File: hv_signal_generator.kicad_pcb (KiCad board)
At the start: 2 copper layers, 83.8 x 121.9 mm, 210 parts, among them IC1 ATMEG328PU, J1 CONN_4, J2 CONN_10, J3 CONN_2, J4 CONN_2, J5 CONN_40, P1 CONN_6, P2 CONN_6, SW1 DPST, U1 74HC595A, U2 74HC595A, U3 74HC595A, U4 74HC595A, U5 74HC595A, U6 7400, X1 16MHz

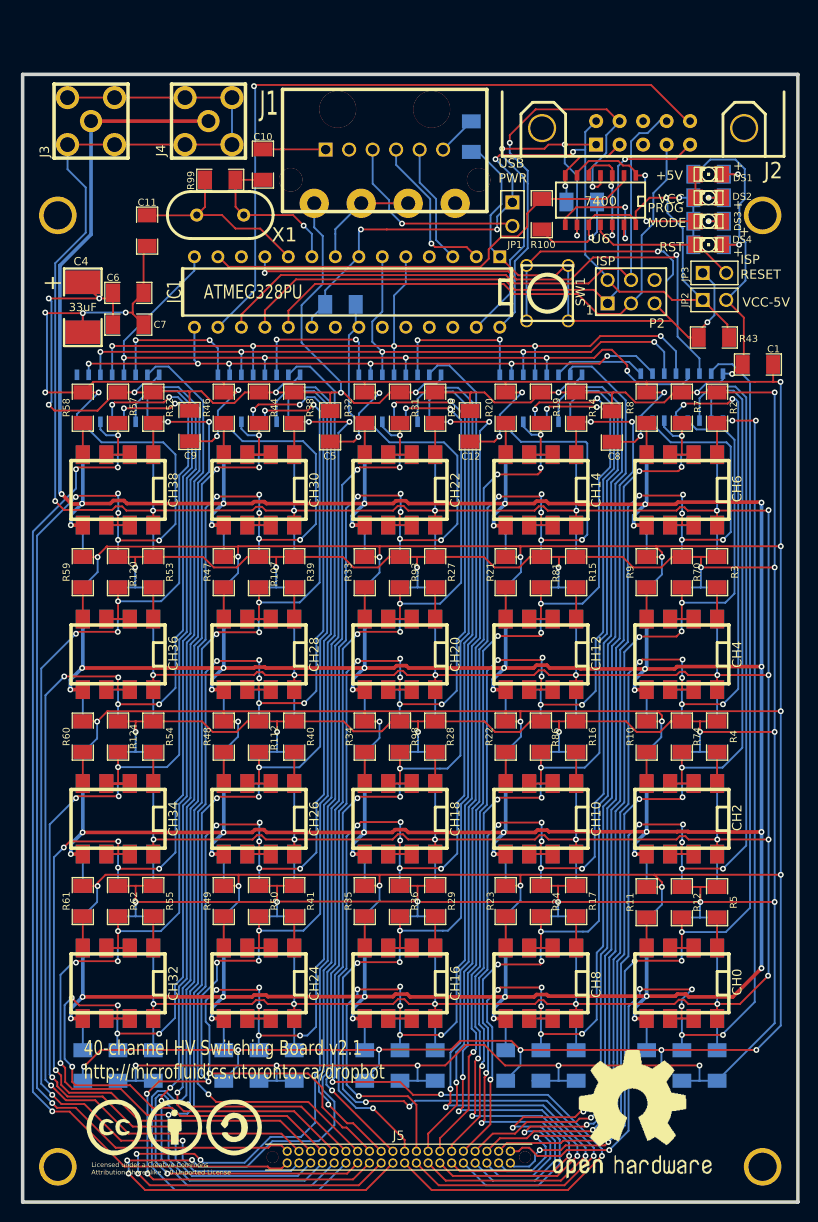
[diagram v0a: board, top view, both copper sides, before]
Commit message: Complete layout
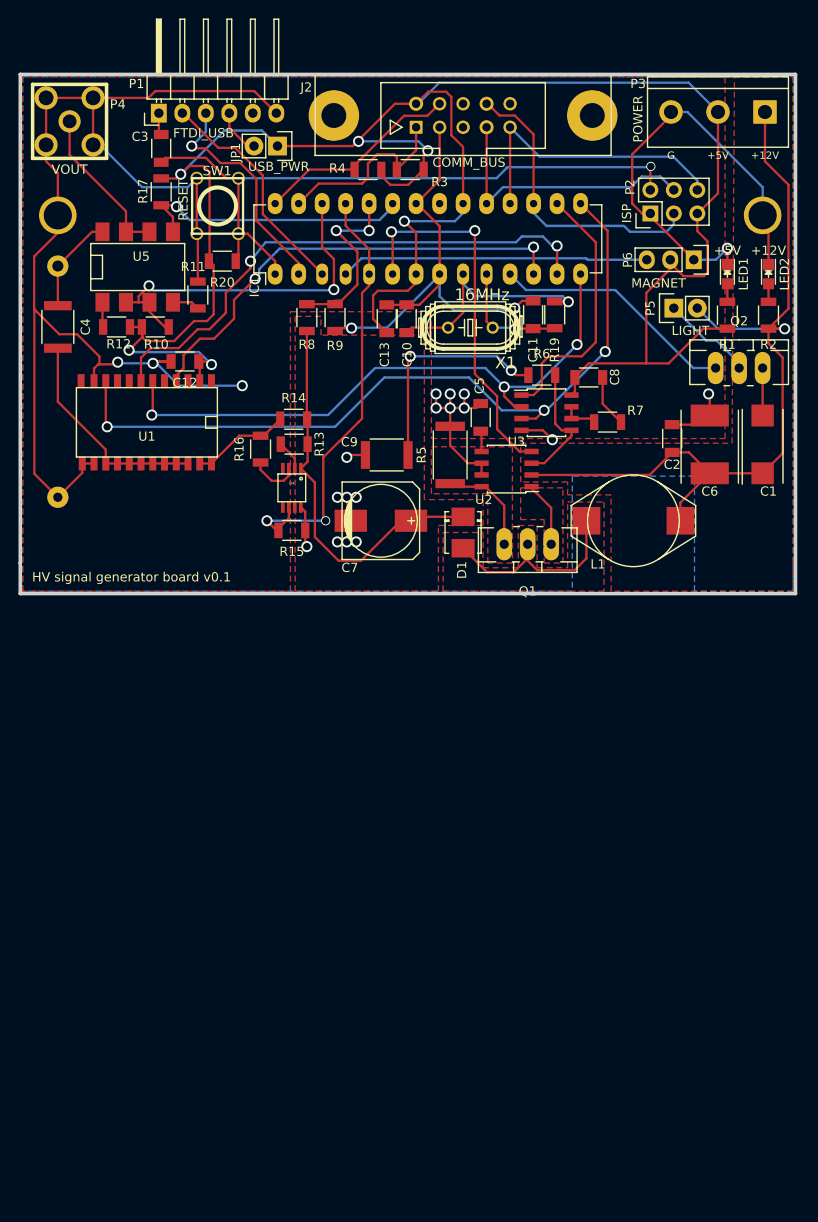
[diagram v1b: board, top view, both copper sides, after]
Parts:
- removed the 1PIN at (20.3, 133.3)
- removed the 1PIN at (96.5, 133.3)
- removed C14: 0.1uF, SM1206
- removed CH0, CH1, CH10, CH11, CH12, CH13, CH14, CH15, CH16, CH17, CH18, CH19, CH2, CH20, CH21, CH22, CH23, CH24, CH25, CH26, CH27, CH28, CH29, CH3, CH30, CH31, CH32, CH33, CH34, CH35, CH36, CH37, CH38, CH39, CH4, CH5, CH6, CH7, CH8, CH9: AQW216, 8DIPCMS
- removed DS1: +5V, LED-1206
- removed DS2: VCC, LED-1206
- removed DS3: PROG_MODE, LED-1206
- removed DS4: RST, LED-1206
- removed G***: LOGO, CC_A_SA_LOGO
- removed G***: LOGO, OSHWLOGO0.75IN
- removed J1: CONN_4, Molex_15-24-4441
- removed J3, J4: CONN_2, JACK_SMA
- removed J5: CONN_40, TFML-120-01-XXX-D-RA
- removed JP2: JUMPER, PIN_ARRAY_2X1
- removed JP3: ISP RESET, PIN_ARRAY_2X1
- removed R100, R125, R126, R127, R45: 1k, SM1206
- removed R101, R106, R107, R112, R114, R118, R120, R124, R24, R25, R30, R31, R36, R37, R42, R44, R50, R51, R56, R57, R62, R64, R68, R70, R74, R75, R80, R81, R86, R87, R92, R93, R98: 4.75k, SM1206
- removed R102, R103, R104, R105, R108, R109, R110, R111, R113, R115, R116, R117, R119, R121, R122, R123, R21, R22, R23, R26, R27, R28, R29, R32, R33, R34, R35, R38, R39, R40, R41, R46, R47, R48, R49, R52, R53, R54, R55, R58, R59, R60, R61, R63, R65, R66, R67, R69, R71, R72, R73, R76, R77, R78, R79, R82, R83, R84, R85, R88, R89, R90, R91, R94, R95, R96, R97: 375, SM1206
- removed R43: 10k, SM1206
- removed R99: 1Meg, SM1206
- removed U6: 7400, SO14E
- added D1: ES2F, Diodes_SMD:DO-214BA, F.Cu at (64.1, 64.8)
- added L1: 100uH, Inductors:self_cms_we-pd3, F.Cu at (82.5, 63.5)
- added LED1: +5V, LEDs:LED_0805, F.Cu at (92.7, 36.8)
- added LED2: +12V, LEDs:LED_0805, F.Cu at (97.2, 36.8)
- added P3: POWER, Connect:bornier3, F.Cu at (91.7, 19.3)
- added P4: VOUT, footprints:JACK_SMA, F.Cu at (21.6, 20.3)
- added P5: LIGHT, Pin_Headers:Pin_Header_Straight_1x02, F.Cu at (86.9, 40.5)
- added P6: MAGNET, Pin_Headers:Pin_Header_Straight_1x03, F.Cu at (89.1, 35.3)
- added Q1: IRF644PBF, TO_SOT_Packages_THT:TO-220_Neutral123_Vertical_LargePads, F.Cu at (71.1, 66.0)
- added Q2: P16NF06, TO_SOT_Packages_THT:TO-220_Neutral123_Vertical_LargePads, F.Cu at (94.0, 47.0)
- C1: value 0.1uF -> 10uF; footprint SM1206 -> Capacitors_Tantalum_SMD:TantalC_SizeD_EIA-7343_Reflow
- C10, C11, C12, C5, C8: footprint SM1206 -> Capacitors_SMD:C_1206
- C13, C3: footprint SM1206 -> Capacitors_SMD:C_1206; moved to F.Cu
- C2: value 33uF -> 0.1uF; footprint SM2917 -> Capacitors_SMD:C_1206; moved to F.Cu
- C4: value 33uF -> 0.1uF; footprint SM2917 -> Capacitors_SMD:C_1812
- C6: value 0.1uF -> 100uF,35V; footprint SM1206 -> Capacitors_Tantalum_SMD:TantalC_SizeE_EIA-7360_Reflow
- C7: value 0.01uF -> 4u7,250V; footprint SM1206 -> Capacitors_SMD:c_elec_8x10.5
- C9: value 0.1uF -> 100nF,250V; footprint SM1206 -> Capacitors_SMD:C_1812
- IC1: footprint DIP-28 -> Housings_DIP:DIP-28_W7.62mm_LongPads
- J2: value CONN_10 -> COMM_BUS; footprint HE10-10C -> Connect:he10-10d
- JP1: value JUMPER -> USB_PWR; footprint PIN_ARRAY_2X1 -> Pin_Headers:Pin_Header_Straight_1x02
- P1: value CONN_6 -> FTDI_USB; footprint PIN_ARRAY-6X1 -> Pin_Headers:Pin_Header_Angled_1x06; moved to F.Cu
- P2: value CONN_6 -> ISP; footprint pin_array_3x2 -> Pin_Headers:Pin_Header_Straight_2x03
- R1: value 4.75k -> 1k; footprint SM1206 -> Resistors_SMD:R_1206; moved to F.Cu
- R10: value 375 -> 4.75k; footprint SM1206 -> Resistors_SMD:R_1206
- R11: footprint SM1206 -> Resistors_SMD:R_1206
- R12: value 4.75k -> 375; footprint SM1206 -> Resistors_SMD:R_1206
- R13: value 4.75k -> 5k; footprint SM1206 -> Resistors_SMD:R_1206; moved to F.Cu
- R14: value 375 -> 5; footprint SM1206 -> Resistors_SMD:R_1206
- R15, R17: value 375 -> 50k; footprint SM1206 -> Resistors_SMD:R_1206
- R16: value 375 -> 100k; footprint SM1206 -> Resistors_SMD:R_1206
- R18: value 4.75k -> 10k; footprint SM1206 -> Resistors_ThroughHole:Resistor_Horizontal_RM25mm
- R19: value 4.75k -> 1Meg; footprint SM1206 -> Resistors_SMD:R_1206
- R2: value 375 -> 2k; footprint SM1206 -> Resistors_SMD:R_1206
- R20: value 375 -> 10k; footprint SM1206 -> Resistors_SMD:R_1206
- R3, R4: value 375 -> 5.1k; footprint SM1206 -> Resistors_SMD:R_1206
- R5: value 375 -> 50m; footprint SM1206 -> Resistors_SMD:R_2512
- R6: value 4.75k -> 2M; footprint SM1206 -> Resistors_SMD:R_1206; moved to F.Cu
- R7: value 4.75k -> 10k; footprint SM1206 -> Resistors_SMD:R_1206
- R8: value 375 -> 2M; footprint SM1206 -> Resistors_SMD:R_1206
- R9: value 375 -> 40k; footprint SM1206 -> Resistors_SMD:R_1206
- SW1: value DPST -> RESET; footprint SW_PUSH_6mm -> footprints:SW_PUSH_6mm
- U1: value 74HC595A -> HV513; footprint SO16E -> footprints:SOW-24; moved to F.Cu
- U2: value 74HC595A -> MAX1771; footprint SO16E -> Housings_SOIC:SOIC-8_3.9x4.9mm_Pitch1.27mm; moved to F.Cu
- U3: value 74HC595A -> MCP41050; footprint SO16E -> Housings_SOIC:SOIC-8_3.9x4.9mm_Pitch1.27mm; moved to F.Cu
- U4: value 74HC595A -> HV7802; footprint SO16E -> footprints:MSOP-8; moved to F.Cu
- U5: value 74HC595A -> AQW216; footprint SO16E -> SMD_Packages:DIP-8_SMD; moved to F.Cu
- X1: footprint HC-49V -> footprints:SparkFun-HC49U-V
- moved R17 88.8 mm to (31.5, 27.9), turned to 270 degrees
- moved R12 87.2 mm to (26.7, 42.5), turned to 0 degrees
- moved R11 81.6 mm to (35.5, 39.1)
- moved R4 72.0 mm to (53.8, 25.5), turned to 180 degrees
- moved R10 69.2 mm to (30.9, 42.5), turned to 0 degrees
- moved C2 65.3 mm to (86.7, 54.6), turned to 90 degrees
- moved C6 65.0 mm to (90.8, 55.2), turned to 90 degrees
- moved R1 63.7 mm to (92.7, 41.3)
- moved R18 58.3 mm to (20.3, 61.0)
- moved U1 57.9 mm to (29.9, 52.9)
- moved R5 56.3 mm to (62.7, 56.4)
- moved R13 56.1 mm to (45.9, 55.2), turned to 180 degrees
- moved R3 54.7 mm to (58.4, 25.5), turned to 180 degrees
- moved R16 46.2 mm to (42.2, 55.8)
- moved R9 43.5 mm to (50.3, 41.5), turned to 90 degrees
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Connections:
- 1PIN pad 1: (no net) -> GND (x2)
- C1 pad 1: +5V -> +12V
- C10 pad 2: N-00000116 -> Net-(C10-Pad2)
- C11 pad 2: N-00000127 -> Net-(C11-Pad2)
- C13 pad 2: VCC -> +5V
- C2 pad 1: +5V -> +12V
- C3 pad 1: N-00000115 -> Net-(C3-Pad1)
- C4 pad 1: +5V -> VOUT
- C4 pad 2: GND -> Net-(C4-Pad2)
- C5 pad 1: +5V -> Net-(C5-Pad1)
- C6 pad 1: +5V -> +12V
- C7 pad 1: +5V -> Net-(C7-Pad1)
- C8 pad 1: +5V -> GND
- C8 pad 2: GND -> +5V
- C9 pad 1: +5V -> Net-(C7-Pad1)
- IC1 pad 10: N-00000127 -> Net-(C11-Pad2)
- IC1 pad 11: D5/S_MOSI -> D5/LED
- IC1 pad 12: (no net) -> D6/BL
- IC1 pad 13: D7 -> D7/HV513_CS
- IC1 pad 14: D8/OE -> D8/S_SCK
- IC1 pad 15: D9/SRCLR -> D9/S_MOSI
- IC1 pad 16: D10/SS -> D10/MCP41050_CS
- IC1 pad 20: VCC -> +5V
- IC1 pad 21: (no net) -> Net-(IC1-Pad21)
- IC1 pad 23: (no net) -> A0/SHORT_CHK
- IC1 pad 24: (no net) -> A1/HV_FB
- IC1 pad 25: (no net) -> D3/A2/CURRENT_SENSE
- IC1 pad 26: (no net) -> A3/OUTPUT_SELECT
- IC1 pad 4: (no net) -> D2/SERVO
- IC1 pad 5: D3/S_SS -> D3/A2/CURRENT_SENSE
- IC1 pad 6: D4/S_SCK -> D4/SHDN
- IC1 pad 7: VCC -> +5V
- IC1 pad 9: N-00000116 -> Net-(C10-Pad2)
- J2 pad 10: D10/SS -> Net-(J2-Pad10)
- J2 pad 2: VCC -> +5V
- J2 pad 5: (no net) -> Net-(J2-Pad5)
- J2 pad 6: (no net) -> Net-(J2-Pad6)
- JP1 pad 1: VCC -> +5V
- P1 pad 1: GND -> Net-(C3-Pad1)
- P1 pad 2: (no net) -> RX
- P1 pad 3: +5V_USB -> TX
- P1 pad 4: TX -> +5V_USB
- P1 pad 5: RX -> Net-(P1-Pad5)
- P1 pad 6: N-00000115 -> GND
- P2 pad 1: D12/MISO -> GND
- P2 pad 2: VCC -> RST
- P2 pad 3: D13/SCK -> D11/MOSI
- P2 pad 4: D11/MOSI -> D13/SCK
- P2 pad 5: RST -> +5V
- P2 pad 6: GND -> D12/MISO
- R1 pad 2: OUT3 -> Net-(LED1-Pad2)
- R10 pad 1: GND -> +5V
- R10 pad 2: N-00000187 -> A3/OUTPUT_SELECT
- R11 pad 2: N-00000195 -> Net-(R11-Pad2)
- R12 pad 1: +5V -> Net-(R12-Pad1)
- R12 pad 2: OUT0 -> +5V
- R13 pad 1: +5V -> Net-(C7-Pad1)
- R13 pad 2: OUT11 -> Net-(R13-Pad2)
- R14 pad 1: N-00000184 -> HV
- R14 pad 2: +5V -> Net-(C7-Pad1)
- R15 pad 1: N-00000183 -> GND
- R15 pad 2: +5V -> D3/A2/CURRENT_SENSE
- R16 pad 1: N-00000174 -> Net-(R16-Pad1)
- R16 pad 2: +5V -> HV
- R17 pad 1: N-00000207 -> +5V
- R17 pad 2: +5V -> A0/SHORT_CHK
- R18 pad 1: +5V -> GND
- R18 pad 2: OUT13 -> VOUT
- R19 pad 1: +5V -> Net-(C10-Pad2)
- R19 pad 2: OUT14 -> Net-(C11-Pad2)
- R2 pad 1: N-00000171 -> +12V
- R2 pad 2: +5V -> Net-(LED2-Pad2)
- R20 pad 1: GND -> RST
- R20 pad 2: N-00000180 -> +5V
- R3 pad 1: N-00000173 -> +5V
- R3 pad 2: +5V -> A4/SDA
- R4 pad 1: N-00000189 -> +5V
- R4 pad 2: +5V -> A5/SCL
- R5 pad 1: N-00000194 -> Net-(Q1-Pad3)
- R5 pad 2: +5V -> GND
- R6 pad 1: +5V -> Net-(C7-Pad1)
- R6 pad 2: OUT5 -> Net-(R6-Pad2)
- R7 pad 1: +5V -> Net-(R7-Pad1)
- R7 pad 2: OUT6 -> GND
- R8 pad 1: GND -> A1/HV_FB
- R8 pad 2: N-00000191 -> Net-(C7-Pad1)
- R9 pad 2: N-00000188 -> A1/HV_FB
- U1 pad 1: OUT1 -> (no net)
- U1 pad 10: D9/SRCLR -> D9/S_MOSI
- U1 pad 11: D4/S_SCK -> GND
- U1 pad 12: D3/S_SS -> (no net)
- U1 pad 13: D8/OE -> GND
- U1 pad 14: D5/S_MOSI -> GND
- U1 pad 15: OUT0 -> Net-(C4-Pad2)
- U1 pad 16: +5V -> Net-(C4-Pad2)
- U1 pad 2: OUT2 -> +5V
- U1 pad 3: OUT3 -> Net-(U1-Pad3)
- U1 pad 4: OUT4 -> D6/BL
- U1 pad 5: OUT5 -> Net-(U1-Pad5)
- U1 pad 6: OUT6 -> D8/S_SCK
- U1 pad 7: OUT7 -> D7/HV513_CS
- U1 pad 8: GND -> Net-(U1-Pad8)
- U1 pad 9: N-0000038 -> Net-(U1-Pad9)
- U2 pad 1: OUT9 -> Net-(Q1-Pad1)
- U2 pad 2: OUT10 -> +12V
- U2 pad 3: OUT11 -> Net-(R6-Pad2)
- U2 pad 4: OUT12 -> D4/SHDN
- U2 pad 5: OUT13 -> Net-(C5-Pad1)
- U2 pad 6: OUT14 -> GND
- U2 pad 7: OUT15 -> GND
- U2 pad 8: GND -> Net-(Q1-Pad3)
- U3 pad 1: OUT17 -> D10/MCP41050_CS
- U3 pad 2: OUT18 -> D8/S_SCK
- U3 pad 3: OUT19 -> D9/S_MOSI
- U3 pad 4: OUT20 -> GND
- U3 pad 5: OUT21 -> Net-(R6-Pad2)
- U3 pad 6: OUT22 -> Net-(R7-Pad1)
- U3 pad 7: OUT23 -> Net-(R7-Pad1)
- U3 pad 8: GND -> +5V
- U4 pad 1: OUT25 -> Net-(C7-Pad1)
- U4 pad 2: OUT26 -> Net-(R13-Pad2)
- U4 pad 3: OUT27 -> Net-(R16-Pad1)
- U4 pad 4: OUT28 -> (no net)
- U4 pad 5: OUT29 -> (no net)
- U4 pad 6: OUT30 -> D3/A2/CURRENT_SENSE
- U4 pad 7: OUT31 -> (no net)
- U5 pad 1: OUT33 -> Net-(R12-Pad1)
- U5 pad 2: OUT34 -> A3/OUTPUT_SELECT
- U5 pad 3: OUT35 -> A3/OUTPUT_SELECT
- U5 pad 4: OUT36 -> Net-(R11-Pad2)
- U5 pad 5: OUT37 -> A0/SHORT_CHK
- U5 pad 6: OUT38 -> Net-(P4-Pad1)
- U5 pad 7: OUT39 -> Net-(P4-Pad1)
- U5 pad 8: GND -> VOUT
- X1 pad 1: N-00000127 -> Net-(C11-Pad2)
- X1 pad 2: N-00000116 -> Net-(C10-Pad2)
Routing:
- net HV: track 597.1 -> 10.9 mm, vias 45 -> 0
- net HVGND: track 569.1 -> 0.00 mm, vias 25 -> 0
- net +5V: track 712.7 -> 231.2 mm, vias 34 -> 6
- net GND: track 728.2 -> 302.4 mm, vias 40 -> 22
- net HVOUT23: track 132.6 -> 0.00 mm, vias 5 -> 0
- net VCC: track 126.4 -> 0.00 mm, vias 7 -> 0
- net HVOUT21: track 120.4 -> 0.00 mm, vias 5 -> 0
- net HVOUT15: track 116.8 -> 0.00 mm, vias 5 -> 0
- net HVOUT39: track 108.9 -> 0.00 mm, vias 3 -> 0
- net HVOUT7: track 106.6 -> 0.00 mm, vias 4 -> 0
- net HVOUT31: track 106.5 -> 0.00 mm, vias 4 -> 0
- net HVOUT38: track 106.4 -> 0.00 mm, vias 4 -> 0
- net HVOUT19: track 97.5 -> 0.00 mm, vias 5 -> 0
- net HVOUT30: track 97.1 -> 0.00 mm, vias 4 -> 0
- net HVOUT29: track 95.3 -> 0.00 mm, vias 2 -> 0
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- added copper zone on F.Cu, net +12V
- added copper zone on F.Cu, net Net-(C7-Pad1)
- added copper zone on F.Cu, net Net-(D1-Pad2)
- added copper zone on F.Cu, net Net-(Q1-Pad1)
- added copper zone on F.Cu, net Net-(Q1-Pad3)
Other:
- board size 83.8 x 121.9 mm -> 83.8 x 56.1 mm
- net class Default: clearance 0.2032 -> 0.4; trace_width 0.2032 -> 0.254; via_dia 0.635 -> 1.2; via_drill 0.381 -> 0.8
- net class HV removed
- rule trace_clearance: 0.2032 -> 0.4
- board text added: "+12V"
- board text added: "HV signal generator board v0.1"
- board text removed: "+"
- board text removed: "1"
- board text removed: "40-channel HV Switching Board v2.1 http://microfluidics.utoronto.ca/dropbot"
- board text removed: "ISP"
- board text removed: "ISP RESET"
- board text removed: "Licensed under a Creative Commons Attribution-ShareAlike 3.0 Unported License"
- board text removed: "PROG MODE"
- board text removed: "RST"
- board text removed: "USB PWR"
- board text removed: "VCC"
- board text removed: "VCC-5V"
